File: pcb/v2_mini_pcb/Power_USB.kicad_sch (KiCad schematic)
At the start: 37 parts, among them J6 USB4105-GF-A, U10 TPS63802DLAR, U6 TPD4EUSB30, U8 BQ25622ERYKR, U9 MAX17048G_T10

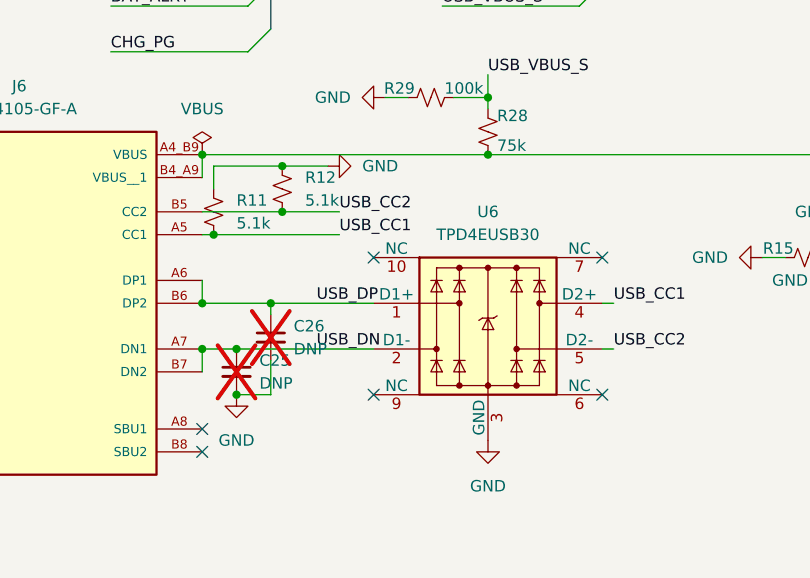
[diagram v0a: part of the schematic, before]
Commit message: vbus connection
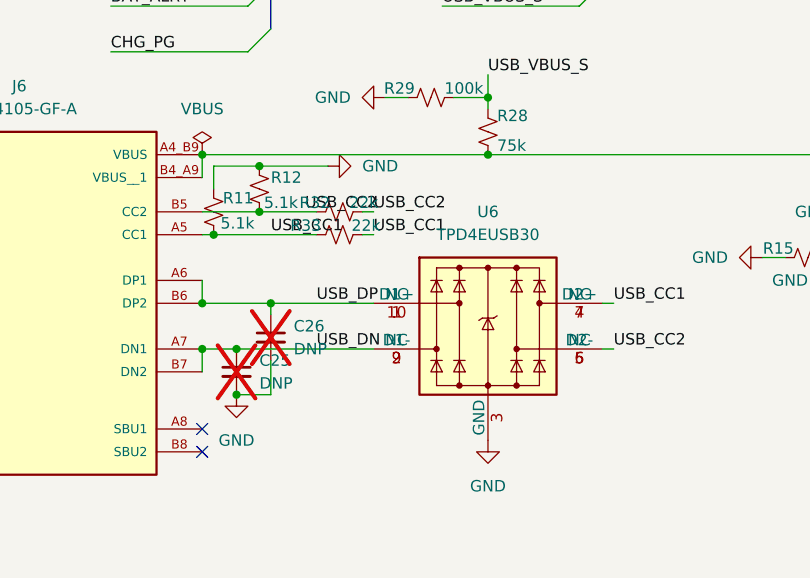
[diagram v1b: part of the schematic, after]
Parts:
- added R32, R33: 22k, Resistor_SMD:R_0402_1005Metric, symbol Device:R_Small_US
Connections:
- net USB_CC1: now also U6.7 (NC), R33.1, R33.2
- net USB_CC2: now also U6.6 (NC), R32.1, R32.2
- net USB_DN: now also U6.9 (NC)
- net USB_DP: now also U6.10 (NC)
- no-connect marks 8 -> 4
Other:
- moved on the sheet: R12
